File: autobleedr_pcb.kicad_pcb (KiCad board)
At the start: 4 copper layers, 126.4 x 105.2 mm, 45 parts, among them J11 Conn_01x02_Pin, J13 Screw_Terminal_01x08, J7 Screw_Terminal_01x02, Q1 PMOS, Q2 IRLML2060, SW1 SW_SPST, U2 ESP32, U6 TMC2209

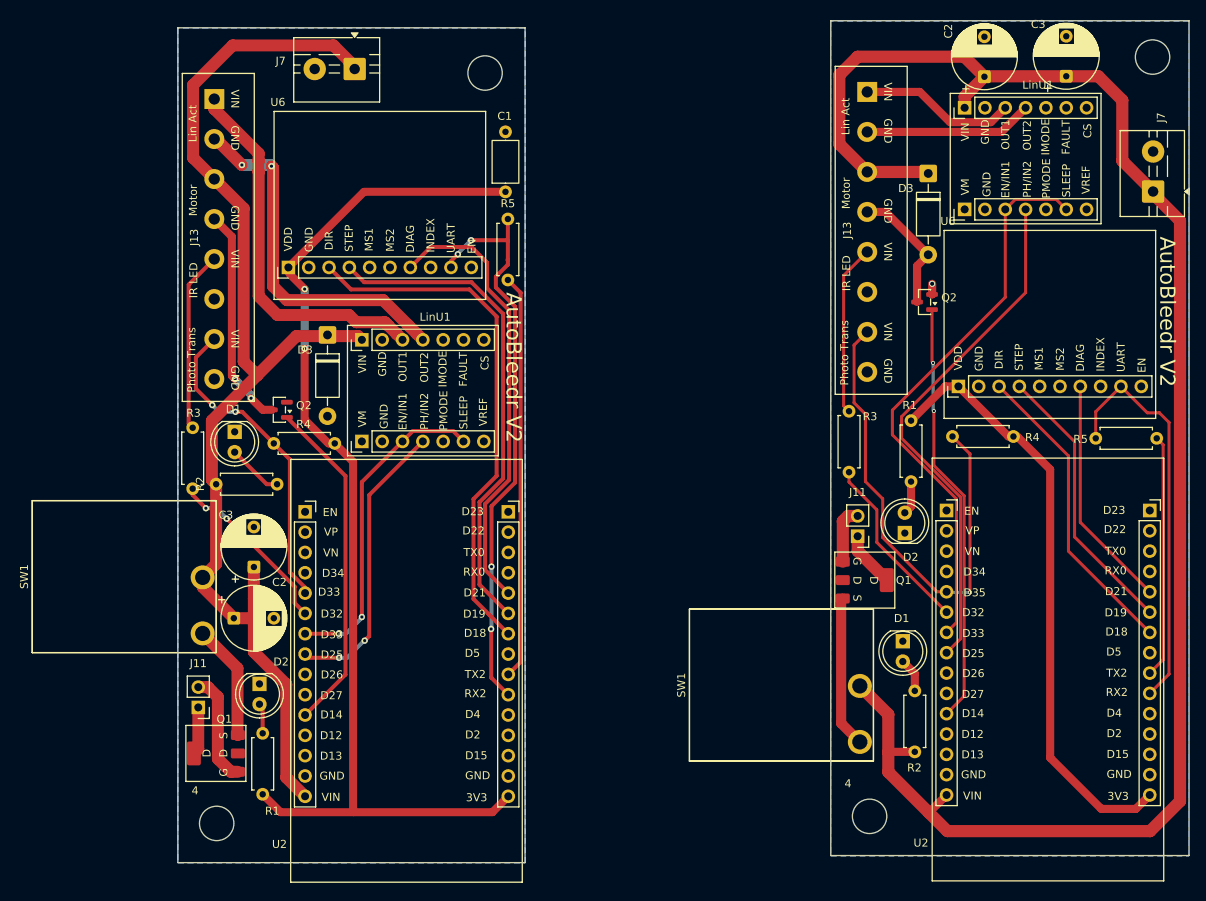
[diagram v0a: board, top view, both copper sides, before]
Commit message: Redid pcb
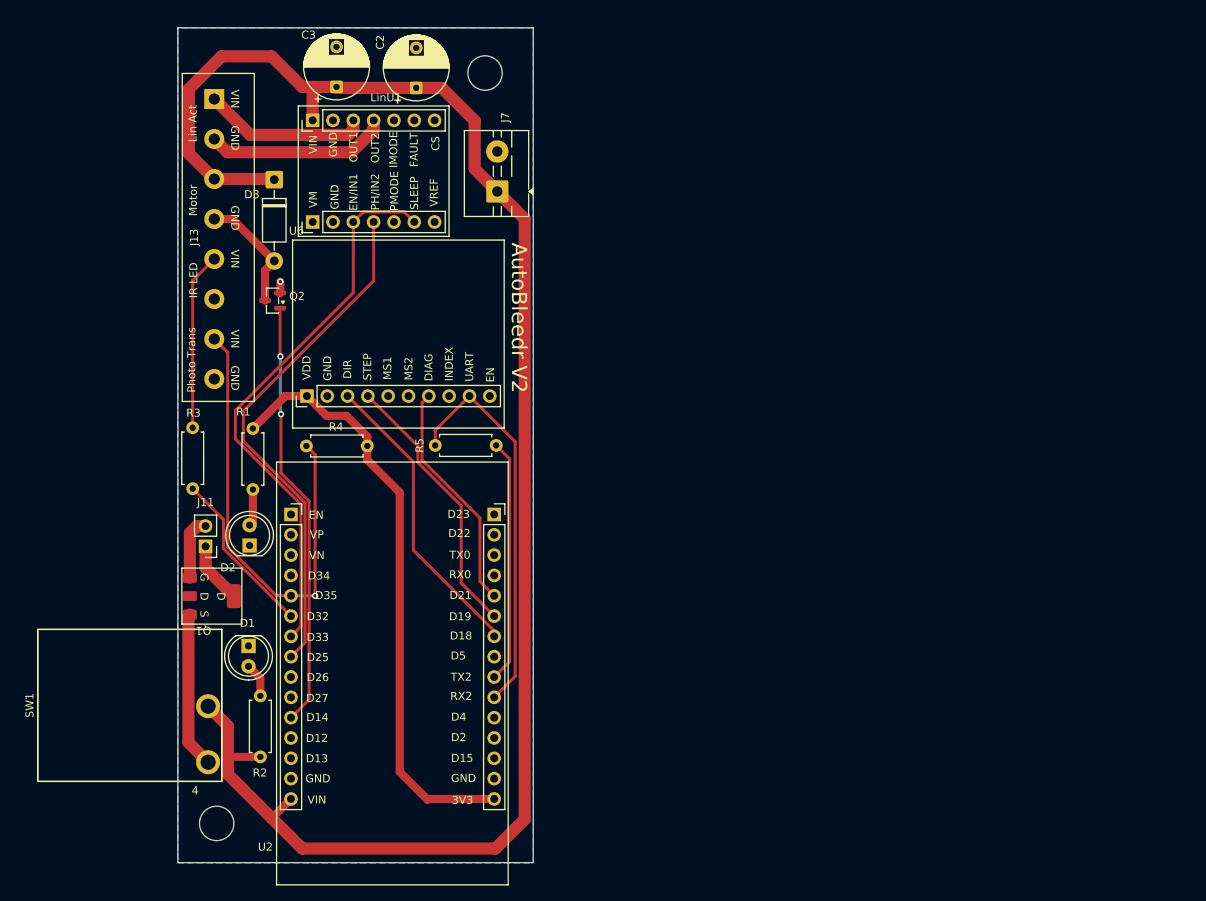
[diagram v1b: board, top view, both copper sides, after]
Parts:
- removed the 2 at (170.8, 76.3)
- removed the 4 at (135.5, 171.2)
- removed the ? at (190.7, 111.3)
- removed C1: 0u1C, Capacitor_THT:C_Axial_L5.1mm_D3.1mm_P7.50mm_Horizontal
- removed the C2 at (149.8, 78.7)
- removed the C3 at (160.0, 78.7)
- removed the D1 at (139.6, 149.3)
- removed the D2 at (139.9, 135.8)
- removed the D3 at (142.8, 90.8)
- removed the J11 at (134.0, 136.2)
- removed the J13 at (136.2, 97.9)
- removed the J7 at (170.9, 93.1)
- removed the LinU1 at (145.5, 88.8)
- removed the Q1 at (135.1, 141.6)
- removed the Q2 at (142.3, 106.9)
- removed the R1 at (140.6, 129.3)
- removed the R2 at (141.1, 155.5)
- removed the R3 at (132.9, 128.1)
- removed the R4 at (153.4, 123.7)
- removed the R5 at (171.4, 123.9)
- removed the SW1 at (123.9, 154.8)
- removed the U2 at (145.2, 132.9)
- removed the U6 at (157.9, 109.9)
- moved C2 70.1 mm to (78.8, 80.1), turned to 90 degrees
- moved C3 60.9 mm to (68.8, 80.0)
- moved R1 30.5 mm to (58.4, 130.3), turned to 90 degrees
- moved LinU1 28.1 mm to (64.0, 90.4)
- moved D1 26.8 mm to (57.8, 149.9)
- moved R2 26.5 mm to (59.3, 156.1), turned to -90 degrees
- moved J7 23.5 mm to (88.9, 93.1), turned to 90 degrees
- moved R5 20.7 mm to (88.8, 124.8), turned to 180 degrees
- moved D3 20.5 mm to (61.0, 91.6)
- moved J11 20.2 mm to (52.5, 137.4)
- moved Q1 19.7 mm to (53.5, 143.6), turned to -90 degrees
- moved D2 17.3 mm to (58.0, 137.3), turned to 90 degrees
- moved U6 16.2 mm to (76.5, 111.1)
- moved SW1 16.1 mm to (42.5, 157.3)
- moved Q2 13.7 mm to (60.8, 106.7)
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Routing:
- net +7.5V: track 363.0 -> 214.5 mm
- net +3.3V: track 210.7 -> 75.0 mm, vias 2 -> 0
- net /TMC UART: track 123.2 -> 49.1 mm, vias 4 -> 0
- net /DIR: track 105.2 -> 37.6 mm
- net /STEP: track 96.7 -> 34.0 mm
- net /DIAG: track 85.6 -> 29.0 mm
- net Net-(U2-TX2): track 81.0 -> 30.4 mm
- net /LIN ACT VIN: track 66.8 -> 20.7 mm
- net /LIN ACT GND: track 66.2 -> 23.0 mm, vias 2 -> 0
- net D35: track 102.1 -> 59.3 mm, vias 3 -> 1
- net /speed ERM DRV: track 95.4 -> 53.6 mm
- net /enable DRV: track 112.0 -> 70.5 mm, vias 2 -> 0
- net /linear actuator direction: track 102.1 -> 65.0 mm, vias 2 -> 0
- net /ERM neg: track 43.8 -> 15.1 mm, vias 2 -> 0
- net D32: track 45.2 -> 21.0 mm, vias 2 -> 0
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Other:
- board size 126.4 x 105.2 mm -> 44.4 x 104.3 mm
- board text added: "D35"
- board text removed: "D33"
